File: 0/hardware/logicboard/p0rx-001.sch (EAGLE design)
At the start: 23 parts, among them IC1 74ALS05N, IC2 LTC485N, IC3 LTC485N, IC4 LTC485N, J0 DC5V, J7 DIN5, J8 DIN5, J9 DIN5, X7 NELTRON-7810-XPXC

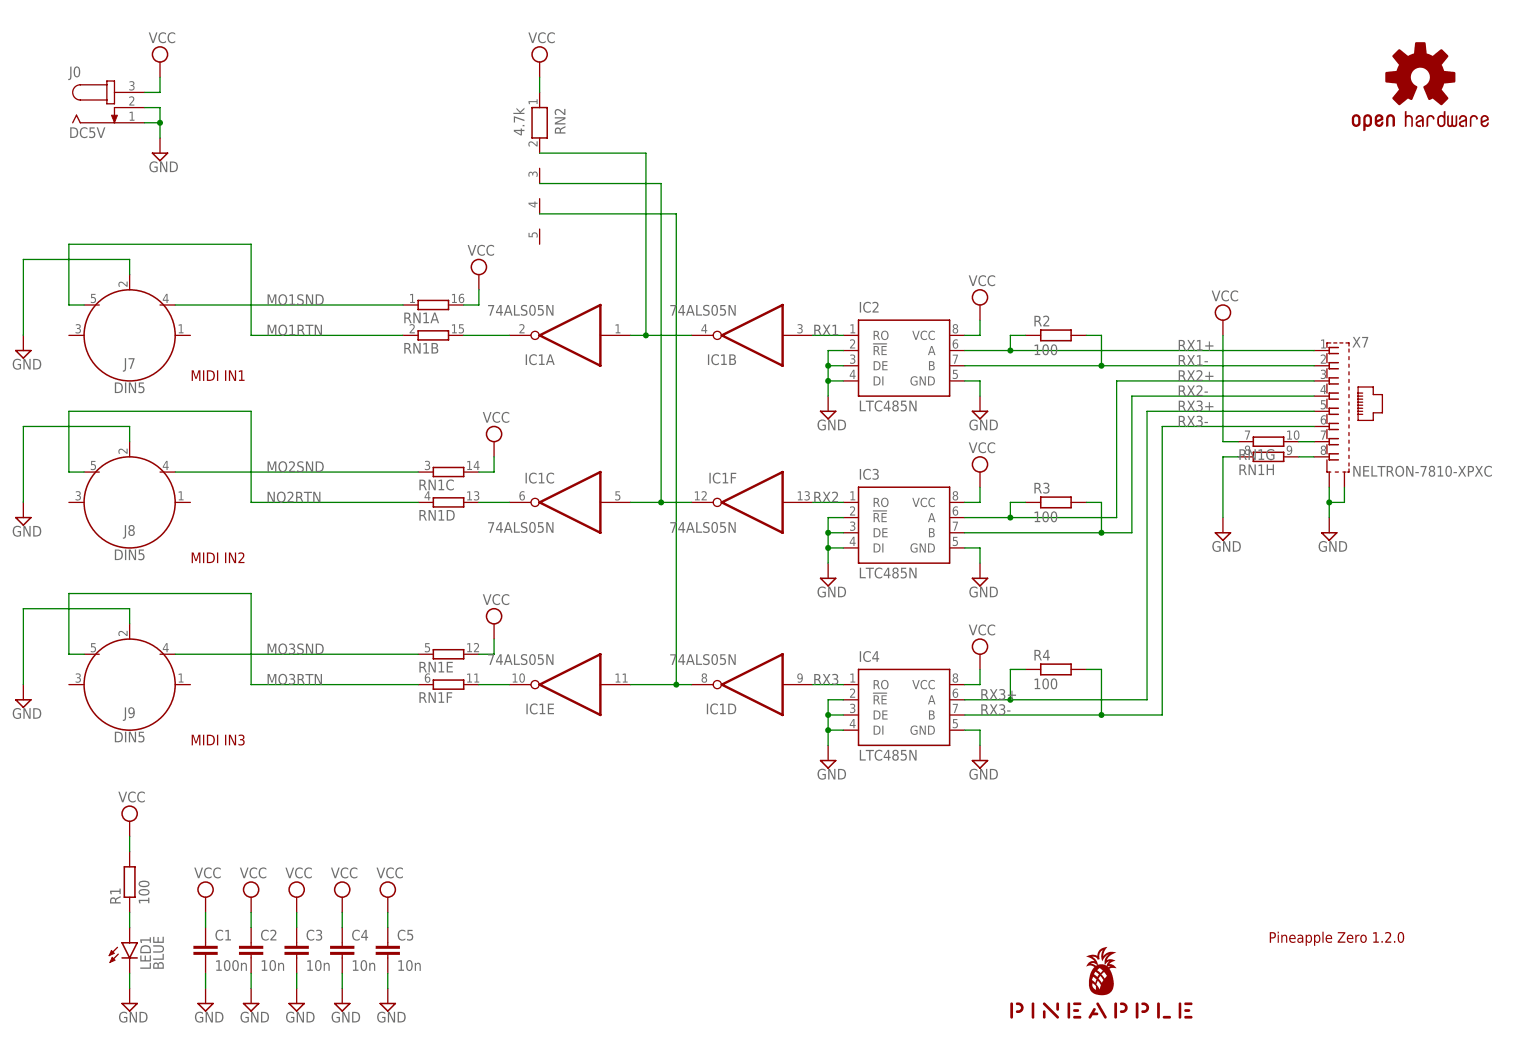
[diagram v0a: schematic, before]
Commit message: Redesign.
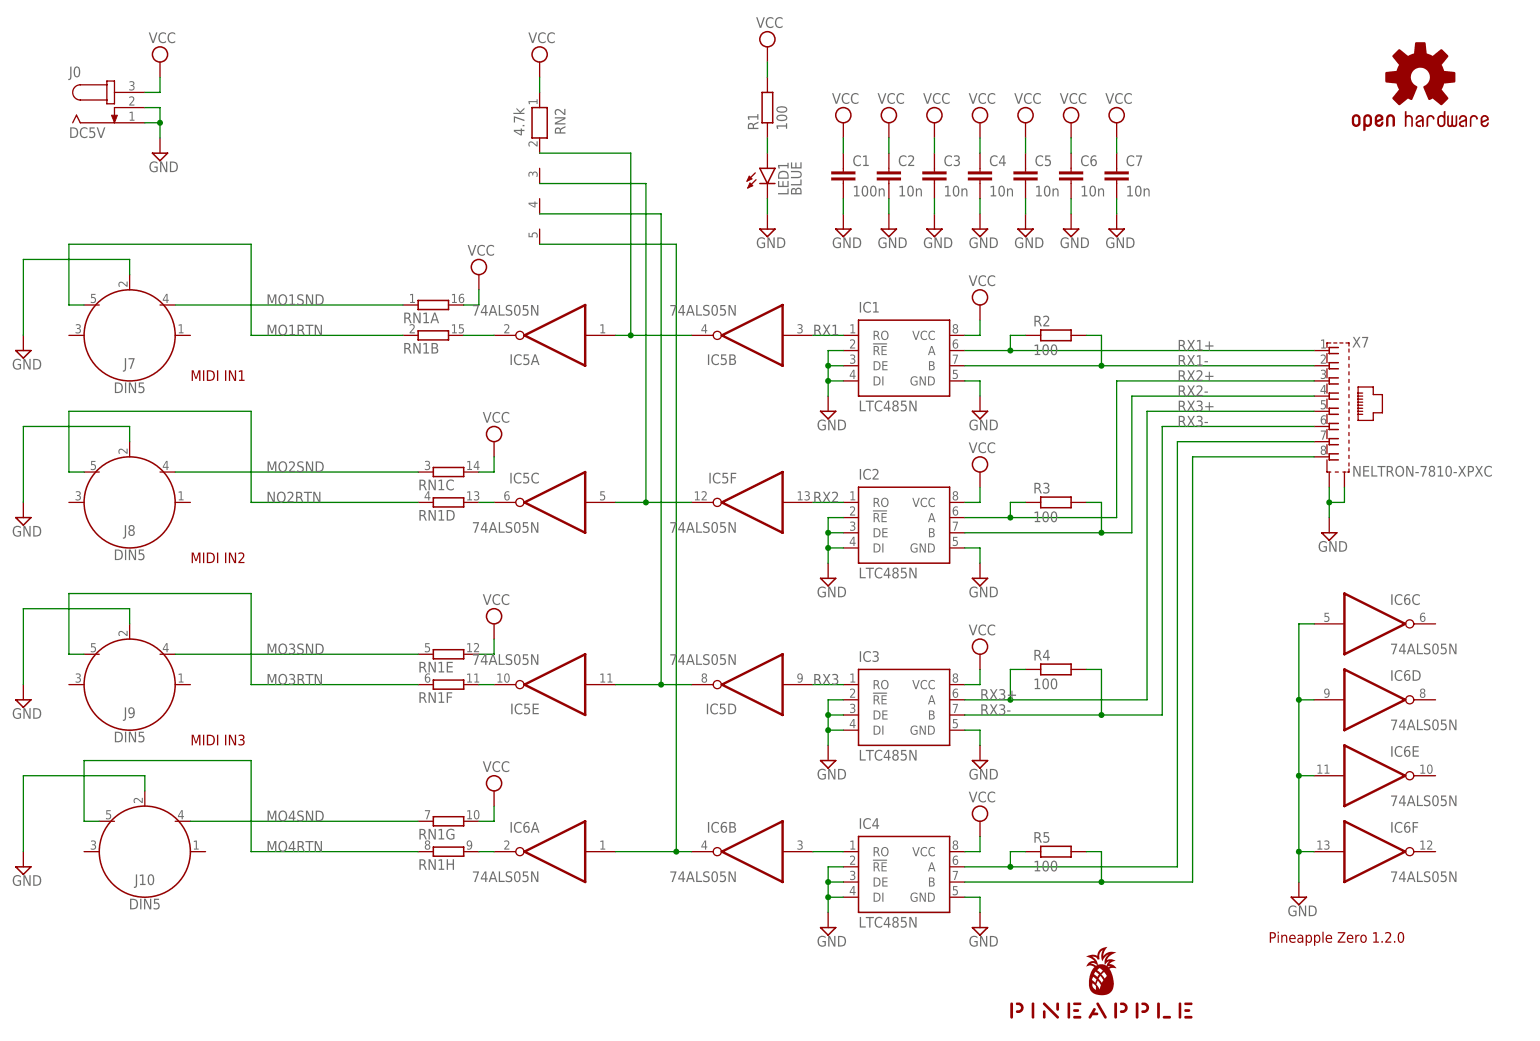
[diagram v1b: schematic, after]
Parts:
- added C6, C7: 10n, rcl:C-EU025-024X044
- added IC5, IC6: 74ALS05N, 74xx-us:74ALS05N
- added J10: DIN5, SparkFun-Connectors:DIN5
- added R5: 100, rcl:R-EU_0204/5
- IC1: value 74ALS05N -> LTC485N; device 74xx-us:74ALS05N -> linear-technology:LTC485N
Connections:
- removed net MNTRRTN: RN1H.2, X7.8
- removed net MNTRSND: RN1G.2, X7.7
- new net MO4RTN: J10.5, RN1H.1
- new net MO4SND: J10.4, RN1G.1
- new net N$1: IC6A.I, IC6B.O, RN2.5
- new net N$2: IC4.RO, IC6B.I
- new net N$3: IC4.A, R5.1, X7.7
- new net N$5: IC4.B, R5.2, X7.8
- new net N$6: IC6A.O, RN1H.2
- net GND: now also C6.2, C7.2, IC1.!RE, IC1.DE, IC1.DI, IC1.GND, IC6C.I, IC6D.I, IC6E.I, IC6F.I, J10.2; no longer RN1H.1
- net MO1RTNRAW: now also IC5A.O; no longer IC1A.O
- net MO2RTNRAW: now also IC5C.O; no longer IC1C.O
- net MO3RTNRAW: now also IC5E.O; no longer IC1E.O
- net RX1: now also IC1.RO, IC5B.I; no longer IC1B.I, IC2.RO
- net RX1+: now also IC1.A; no longer IC2.A
- net RX1-: now also IC1.B; no longer IC2.B
- net RX1R: now also IC5A.I, IC5B.O; no longer IC1A.I, IC1B.O
- net RX2: now also IC2.RO, IC5F.I; no longer IC1F.I, IC3.RO
- net RX2+: now also IC2.A; no longer IC3.A
- net RX2-: now also IC2.B; no longer IC3.B
- net RX2R: now also IC5C.I, IC5F.O; no longer IC1C.I, IC1F.O
- net RX3: now also IC3.RO, IC5D.I; no longer IC1D.I, IC4.RO
- net RX3+: now also IC3.A; no longer IC4.A
- net RX3-: now also IC3.B; no longer IC4.B
- net RX3R: now also IC5D.O, IC5E.I; no longer IC1D.O, IC1E.I
- net VCC: now also C6.1, C7.1, IC1.VCC, RN1G.2; no longer RN1G.1
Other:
- moved on the sheet: C1, C2, C3, C4, C5, IC2, IC3, IC4, LED1, R1, RN1G, RN1H

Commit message: RX indicators.
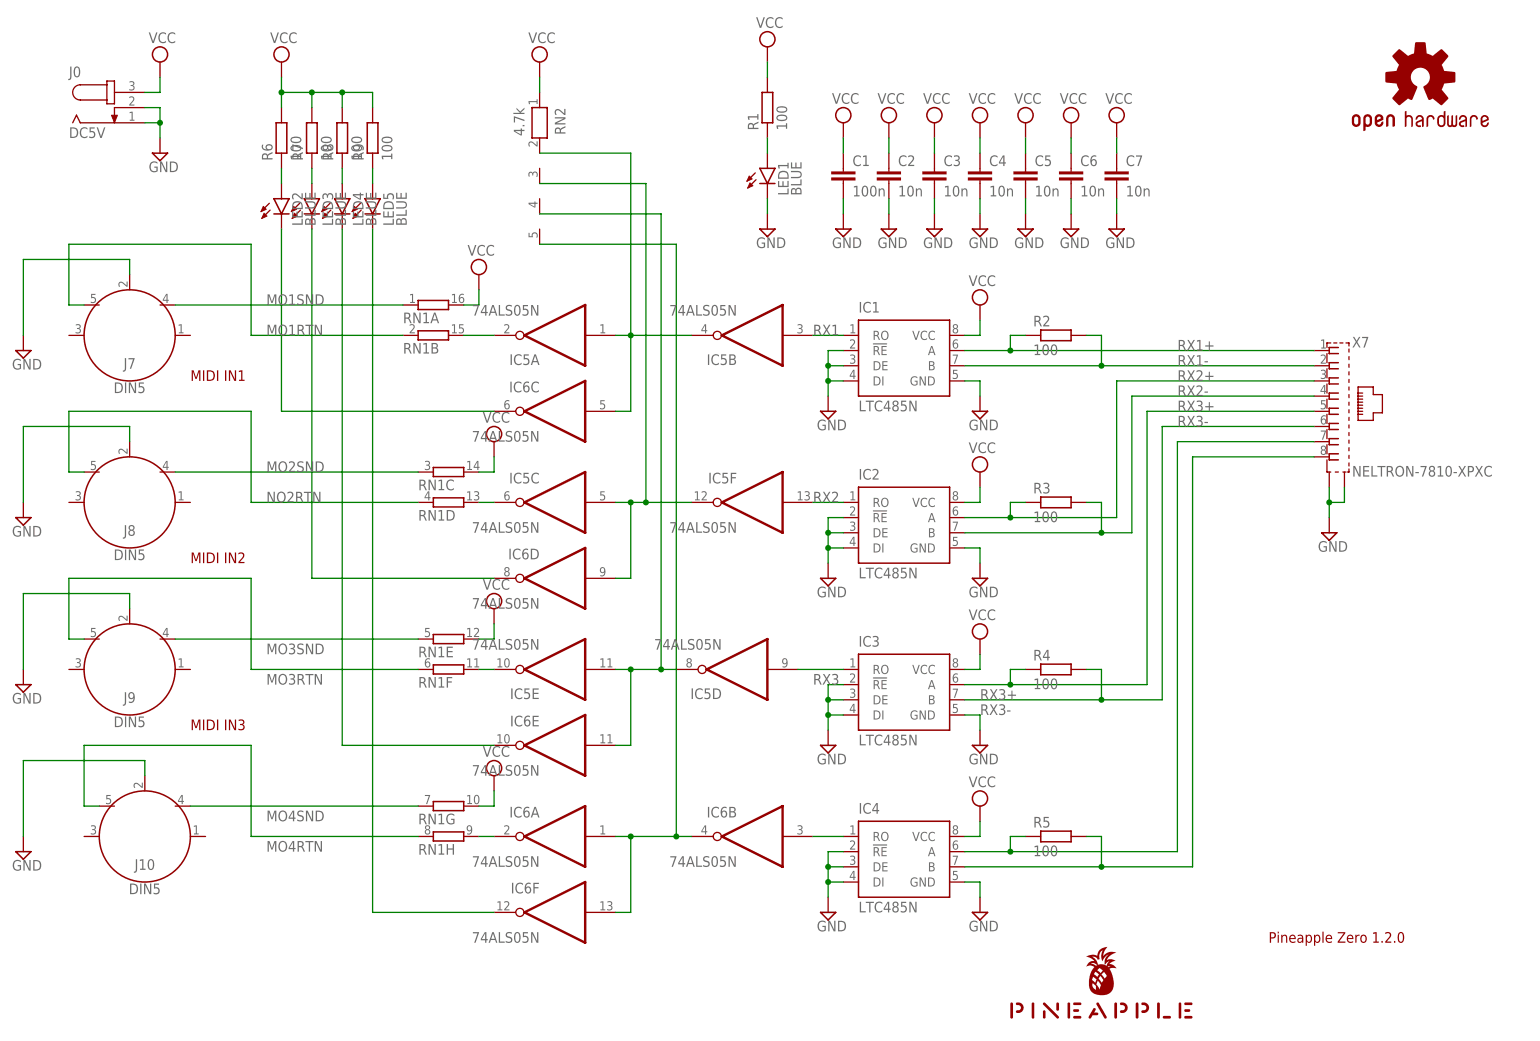
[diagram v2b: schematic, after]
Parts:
- added LED2, LED3, LED4, LED5: BLUE, led:LED3MM
- added R6, R7, R8, R9: 100, rcl:R-EU_0204/5
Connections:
- new net N$10: LED5.A, R9.1
- new net N$11: IC6C.O, LED2.C
- new net N$12: IC6D.O, LED3.C
- new net N$13: IC6E.O, LED4.C
- new net N$14: IC6F.O, LED5.C
- new net N$7: LED2.A, R6.1
- new net N$8: LED3.A, R7.1
- new net N$9: LED4.A, R8.1
- net GND: no longer IC6C.I, IC6D.I, IC6E.I, IC6F.I
- net N$1: now also IC6F.I
- net RX1R: now also IC6C.I
- net RX2R: now also IC6D.I
- net RX3R: now also IC6E.I
- net VCC: now also R6.2, R7.2, R8.2, R9.2
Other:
- moved on the sheet: IC3, IC4, IC5D, IC5E, IC6A, IC6B, IC6C, IC6D, IC6E, IC6F, J10, J9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
